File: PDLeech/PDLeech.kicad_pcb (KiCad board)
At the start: 4 copper layers, 21 parts, among them J1 TYPEC-324DBW-ACP24A, J2 USB_A, P1 U261-241N-4BC2LS, Q1 BSS84, Q2 BSS84, Q3 BSS84, Q4 BSS84, U1 TPS62175DQC

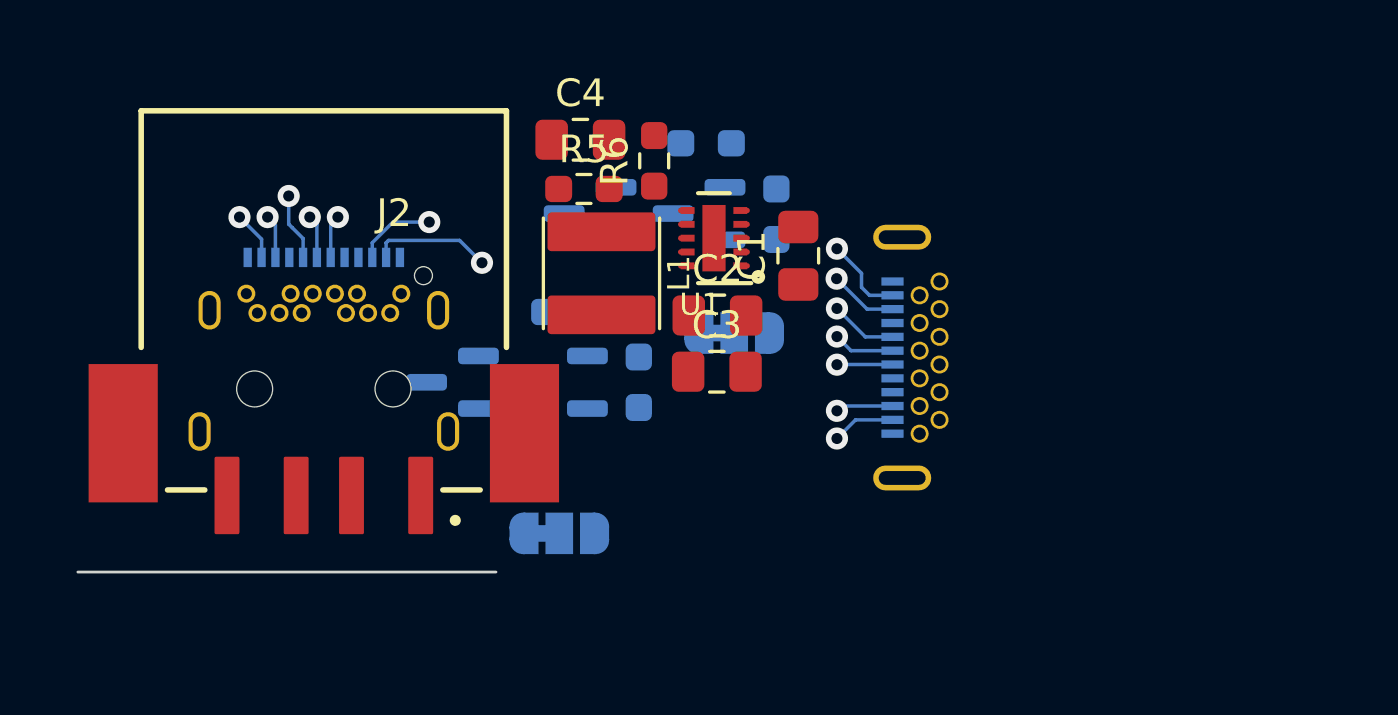
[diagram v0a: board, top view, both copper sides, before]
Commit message: rough layout complete
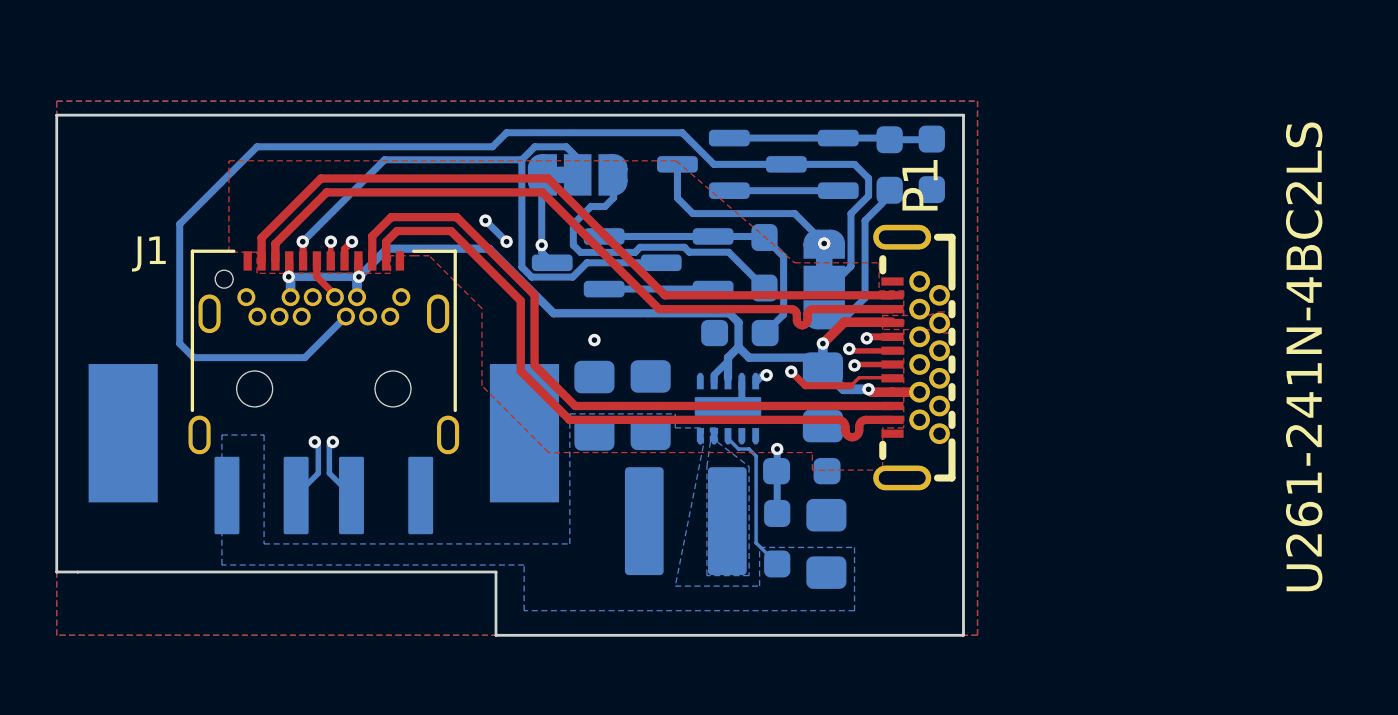
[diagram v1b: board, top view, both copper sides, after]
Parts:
- C1, C2, C3, C4, L1, R5, R6, U1: moved to B.Cu
- J1, P1: moved to F.Cu
- J2: value USB_A -> USB-234-BCW; moved to B.Cu
- moved C4 17.1 mm to (160.1, 73.4), turned to 90 degrees
- moved R5 14.4 mm to (158.4, 73.2), turned to 90 degrees
- moved JP1 13.0 mm to (151.2, 60.1)
- moved R6 12.4 mm to (159.3, 70.8), turned to 0 degrees
- moved L1 9.46 mm to (155.1, 72.6), turned to 180 degrees
- moved R4 8.19 mm to (164.0, 59.7), turned to -90 degrees
- moved Q1 6.27 mm to (151.2, 63.2)
- moved Q2 6.27 mm to (155.1, 63.2)
- moved R1 6.27 mm to (157.9, 63.2)
- moved R2 6.19 mm to (157.0, 65.8)
- moved U1 6.18 mm to (156.6, 68.5), turned to -90 degrees
- moved C1 5.19 mm to (160.0, 68.1), turned to -90 degrees
- moved C3 4.59 mm to (151.8, 68.4), turned to 90 degrees
- moved Q4 4.46 mm to (159.6, 59.7)
- moved Q3 4.46 mm to (155.7, 59.7)
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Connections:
- net Net-(J1-PadA10) renamed /RX2-
- net Net-(J1-PadA11) renamed /RX2+
- net Net-(J1-PadA2) renamed /TX1+
- net Net-(J1-PadA3) renamed /TX1-
- net Net-(J1-PadB10) renamed /RX1-
- net Net-(J1-PadB11) renamed /RX1+
- net Net-(J1-PadB2) renamed /TX2+
- net Net-(J1-PadB3) renamed /TX2-
- J1 pad S1: Net-(J1-PadS1) -> GND
- P1 pad S1: Net-(J1-PadS1) -> GND
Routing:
- net /CC2_OUT: track 0.00 -> 42.7 mm
- net /RX1+: track 0.00 -> 36.0 mm
- net /RX1-: track 0.00 -> 36.0 mm
- net /VBUS: track 0.00 -> 34.7 mm, vias 0 -> 4
- net /TX2-: track 0.00 -> 29.9 mm
- net /TX2+: track 0.00 -> 29.8 mm
- net Net-(J1-PadB8): track 0.00 -> 28.0 mm
- net /CC1_OUT: track 0.00 -> 22.1 mm, vias 0 -> 1
- net /CC1_IN: track 0.00 -> 17.4 mm, vias 0 -> 2
- net /CC2_IN: track 0.00 -> 16.4 mm, vias 0 -> 1
- net /CC1_G: track 0.00 -> 11.1 mm
- net Net-(Q1-Pad1): track 0.00 -> 9.83 mm
- net /D-: track 26.4 -> 35.9 mm, vias 2 -> 3
- net /D+: track 25.2 -> 34.4 mm
- net Net-(Q3-Pad1): track 0.00 -> 7.35 mm
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- added copper zone on B.Cu, net +5V
- added copper zone on F.Cu, net /VBUS
- added copper zone on B.Cu, net GND
- added copper zone on F.Cu, net GND
- added copper zone on In1.Cu, net GND
- added copper zone on In2.Cu, net GND
- added copper zone on B.Cu, net Net-(L1-Pad1)
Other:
- board outline added: 32.8 x 18.8 mm

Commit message: layout done
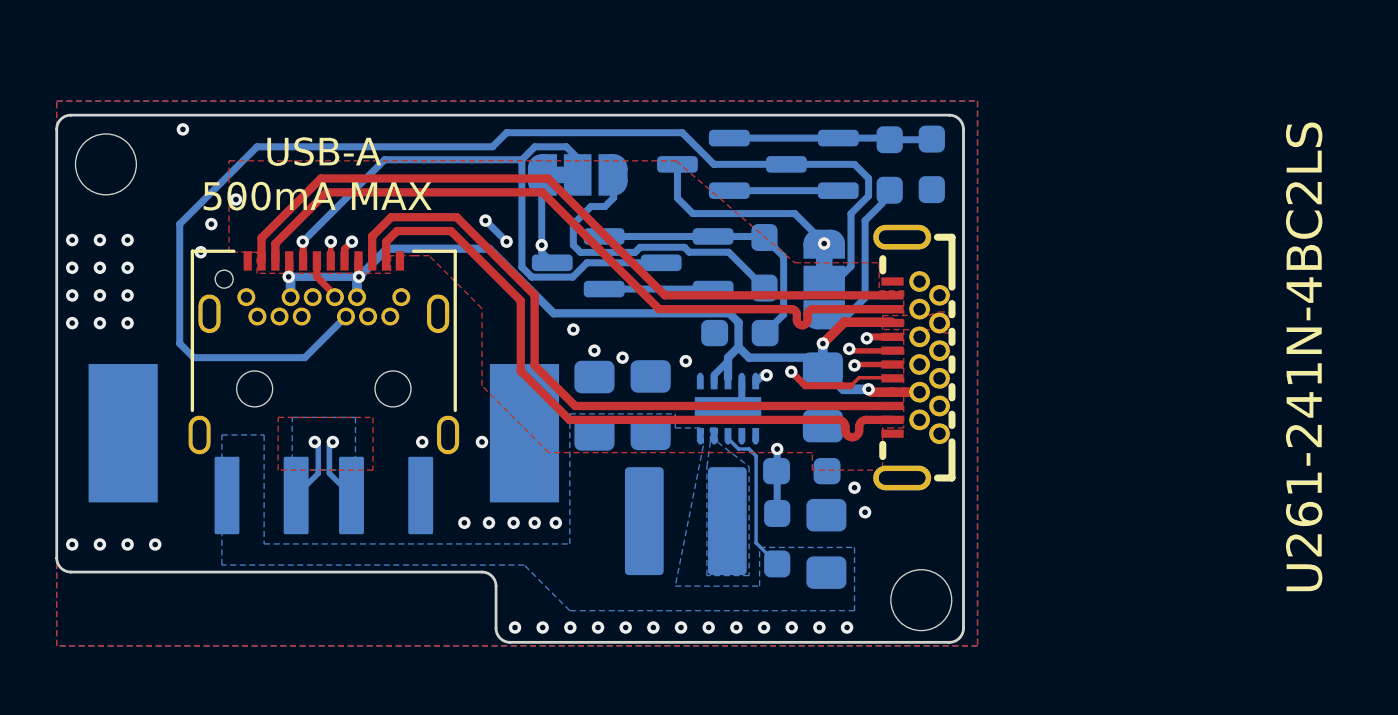
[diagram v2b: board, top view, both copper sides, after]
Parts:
- added REF**: MountingHole_2.2mm_M2, MountingHole:MountingHole_2.2mm_M2, F.Cu at (134.1, 59.7)
- added REF**: MountingHole_2.2mm_M2, MountingHole:MountingHole_2.2mm_M2, F.Cu at (163.6, 75.4)
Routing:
- net GND: vias 1 -> 46
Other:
- board size 32.8 x 18.8 mm -> 32.8 x 19.1 mm
- board text added: "USB-A 500mA MAX"
